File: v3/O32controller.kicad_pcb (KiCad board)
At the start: 4 copper layers, 27 x 27 mm, 89 parts, among them J1 SWD, J12 RS485_2, J14 NTC, J15 ExternalSPI, J2 BATT+, J3 BATT-, J4 Motor Connection, J5 Motor Connection, J6 Motor Connection, J7 BATT+, J8 BATT-, J9 RS485_1, Q1 CSD88584Q5DCT, Q2 CSD88584Q5DCT, Q3 CSD88584Q5DCT, U1 MA702GQ-P, U2 STSPIN32F0A, U3 THVD1420DRLR

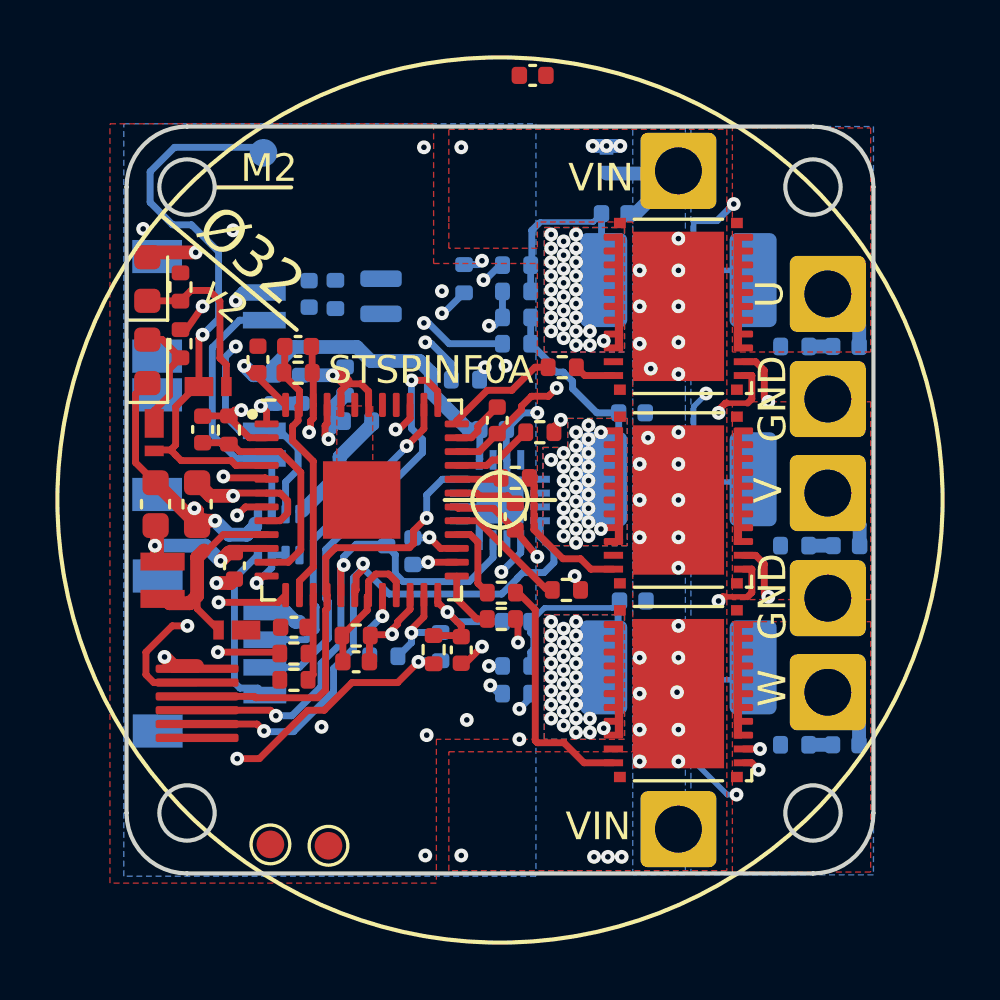
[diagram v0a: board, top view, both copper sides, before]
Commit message: bus caps, finished routing?
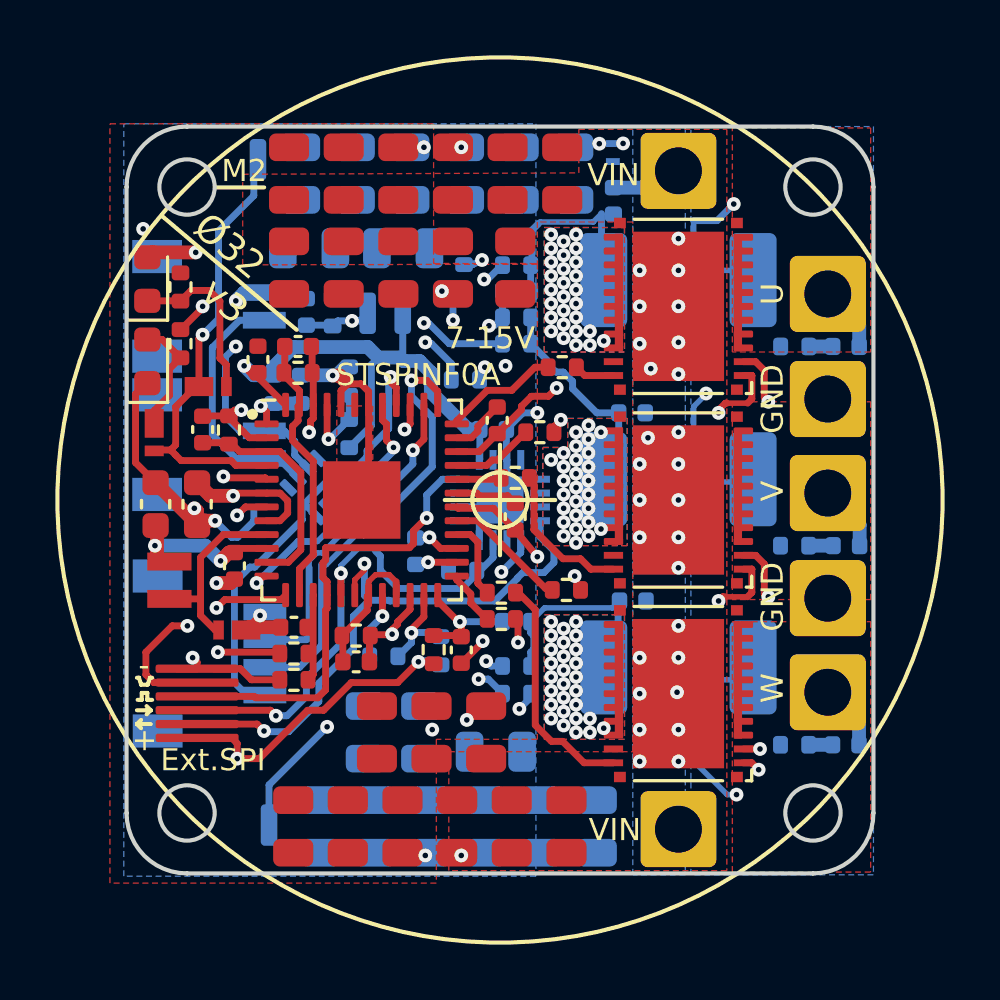
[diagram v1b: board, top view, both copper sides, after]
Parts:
- removed the TP1 at (43.8, 62.5)
- added C21: 22uF, O32controller:C_0805_nosilk, F.Cu at (42.4, 38.2)
- added C22: 22uF, O32controller:C_0805_nosilk, F.Cu at (44.4, 38.2)
- added C23: 22uF, O32controller:C_0805_nosilk, F.Cu at (46.3, 38.2)
- added C24: 22uF, O32controller:C_0805_nosilk, F.Cu at (48.3, 38.2)
- added C25: 22uF, O32controller:C_0805_nosilk, F.Cu at (50.3, 38.2)
- added C26: 22uF, O32controller:C_0805_nosilk, F.Cu at (52.2, 38.2)
- added C27: 22uF, O32controller:C_0805_nosilk, F.Cu at (42.4, 41.6)
- added C28: 22uF, O32controller:C_0805_nosilk, F.Cu at (44.4, 41.6)
- added C29: 22uF, O32controller:C_0805_nosilk, F.Cu at (46.3, 41.6)
- added C30: 22uF, O32controller:C_0805_nosilk, F.Cu at (48.3, 41.6)
- added C31: 22uF, O32controller:C_0805_nosilk, F.Cu at (50.5, 41.6)
- added C32: 22uF, O32controller:C_0805_nosilk, F.Cu at (42.5, 61.8)
- added C33: 22uF, O32controller:C_0805_nosilk, F.Cu at (44.5, 61.8)
- added C34: 22uF, O32controller:C_0805_nosilk, F.Cu at (46.5, 61.8)
- added C35: 22uF, O32controller:C_0805_nosilk, F.Cu at (48.5, 61.8)
- added C36: 22uF, O32controller:C_0805_nosilk, F.Cu at (50.4, 61.8)
- added C37: 22uF, O32controller:C_0805_nosilk, F.Cu at (52.4, 61.8)
- added C38: 22uF, O32controller:C_0805_nosilk, F.Cu at (49.5, 58.4)
- added C39: 22uF, O32controller:C_0805_nosilk, F.Cu at (47.5, 58.4)
- added C41: 22uF, O32controller:C_0805_nosilk, B.Cu at (52.6, 38.2)
- added C42: 22uF, O32controller:C_0805_nosilk, B.Cu at (50.7, 38.2)
- added C43: 22uF, O32controller:C_0805_nosilk, B.Cu at (48.7, 38.2)
- added C44: 22uF, O32controller:C_0805_nosilk, B.Cu at (46.7, 38.2)
- added C45: 22uF, O32controller:C_0805_nosilk, B.Cu at (44.8, 38.2)
- added C46: 22uF, O32controller:C_0805_nosilk, B.Cu at (42.8, 38.2)
- added C47: 22uF, O32controller:C_0805_nosilk, B.Cu at (46.5, 40.9)
- added C48: 22uF, O32controller:C_0805_nosilk, B.Cu at (43.1, 40.9)
- added C49: 22uF, O32controller:C_0805_nosilk, B.Cu at (53.5, 61.8)
- added C50: 22uF, O32controller:C_0805_nosilk, B.Cu at (51.5, 61.8)
- added C51: 22uF, O32controller:C_0805_nosilk, B.Cu at (49.5, 61.8)
- added C52: 22uF, O32controller:C_0805_nosilk, B.Cu at (47.5, 61.8)
- added C53: 22uF, O32controller:C_0805_nosilk, B.Cu at (45.5, 61.8)
- added C54: 22uF, O32controller:C_0805_nosilk, B.Cu at (43.5, 61.8)
- added C55: 22uF, O32controller:C_0805_nosilk, B.Cu at (49.9, 59.1)
- added C56: 22uF, O32controller:C_0805_nosilk, B.Cu at (47.1, 58.4)
- added C57: 22uF, O32controller:C_0805_nosilk, B.Cu at (45.1, 58.4)
- C40: renamed from C8; value 20uF -> 22uF; footprint Capacitor_SMD:C_0402_1005Metric -> O32controller:C_0805_nosilk
- TP1: renamed from TP3; footprint TestPoint:TestPoint_Pad_D1.0mm -> O32controller:TestPoint_Pad_Rect
- TP3: renamed from TP2; footprint TestPoint:TestPoint_Pad_D1.0mm -> O32controller:TestPoint_Pad_Rect; moved to B.Cu
- moved C40 24.4 mm to (45.5, 58.4), turned to 90 degrees
- moved R9 3.09 mm to (48.6, 52.5), turned to 0 degrees
- moved U2 2.20 mm to (43.4, 49.5), turned to 135 degrees
- moved J5 0.79 mm to (46.5, 43.2), turned to 90 degrees
- moved TP3 0.70 mm to (41.6, 61.8), turned to 180 degrees
- moved C9 0.66 mm to (43.0, 43.2), turned to 90 degrees
- moved R7 0.64 mm to (44.0, 43.2), turned to -90 degrees
- moved R32 0.54 mm to (44.5, 47.6), turned to -90 degrees
- moved C12 0.46 mm to (54.1, 39.2), turned to -90 degrees
- moved D2 0.36 mm to (54.1, 37.4)
- moved TP1 0.32 mm to (41.2, 37.7)
- moved L1 0.25 mm to (38.0, 52.9)
- moved R14 0.15 mm to (47.9, 55.5)
- moved R34 0.15 mm to (44.5, 45.7)
- moved C8 0.10 mm to (47.0, 51.9)
- renumbered C7 to C1, C22 to C10, C10 to C11, C18 to C14, C14 to C15, C15 to C16, C19 to C17, C16 to C18, C17 to C19, C1 to C6, C11 to C7, C6 to C8, D4 to D3, D5 to D4, D6 to D5, D3 to D6, J7 to J1, J4 to J10, J5 to J11, J6 to J12, J8 to J4, J14 to J5, J1 to J6, J15 to J7, J9 to J8, J12 to J9, R28 to R1, R27 to R10, R13 to R11, R23 to R12, R15 to R13, R30 to R14, R2 to R15, R31 to R16, R3 to R17, R1 to R18, R4 to R19, R29 to R2, R16 to R20, R24 to R21, R18 to R22, R32 to R23, R6 to R24, R33 to R25, R7 to R26, R5 to R27, R8 to R28, R19 to R29, R14 to R3, R25 to R30, R21 to R31, R34 to R32, R10 to R33, R35 to R34, R11 to R35, R9 to R36, R12 to R37, R22 to R4, R17 to R5, R20 to R6, R36 to R7, R26 to R8, R38 to R9, U2 to U1, U3 to U2, U1 to U3
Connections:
- J7 pad 1: +3.3V -> GND
- J7 pad 6: GND -> +3.3V
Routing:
- net USART_TX: track 6.25 -> 17.3 mm, vias 0 -> 1
- net GND: track 33.8 -> 40.9 mm, vias 24 -> 20
- net /LED_STATUS: track 21.0 -> 16.0 mm
- net /NRST: track 10.2 -> 14.8 mm
- net /USART_RX: track 0.00 -> 3.99 mm, vias 0 -> 1
- net /USART_DE: track 2.20 -> 5.52 mm
- net VBUS: track 28.5 -> 26.5 mm
- net /RS485_B: track 11.2 -> 9.75 mm
- net /OP_W_P: track 16.2 -> 16.9 mm
- net /SPI_MISO: track 18.7 -> 18.1 mm
- net /NTC_IN: track 22.8 -> 23.4 mm, vias 1 -> 2
- net /SPI_MOSI: track 21.6 -> 21.1 mm
- net +3.3V: track 62.8 -> 62.9 mm, vias 8 -> 7
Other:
- board text added: "+"
- board text added: "-"
- board text added: "10k"
- board text added: "7-15V"
- board text added: "D"
- board text added: "Ext.SPI"
- board text added: "JST-SH"
- board text added: "RST"
- board text added: "[12/27/23]"
- board text added: "v3"
- board text removed: "JST"
- board text removed: "SH"
- board text removed: "VIN: 7-15V"
- board text removed: "[1/6/23]"
- board text removed: "v2"
